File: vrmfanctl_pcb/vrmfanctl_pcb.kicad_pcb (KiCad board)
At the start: 2 copper layers, 27.9 x 33.3 mm, 14 parts, among them J1 SATA Power Male, J2 Pin header L-shape, J3 Pin socket L-shape, J4 Pin socket L-shape, Q1 2SC1740, Q2 2SC1740, Q3 2SC1740, U1 ATtiny85-20PU

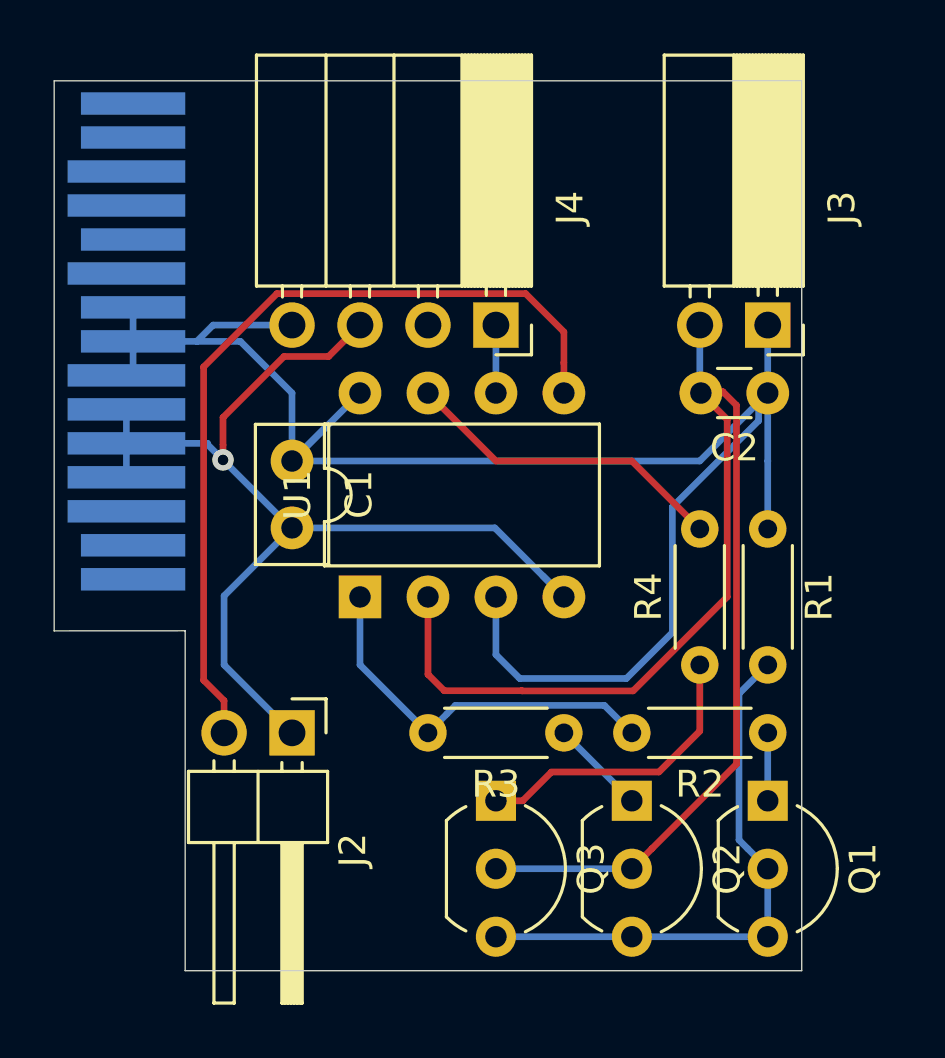
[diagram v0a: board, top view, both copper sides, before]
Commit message: update pcb layout
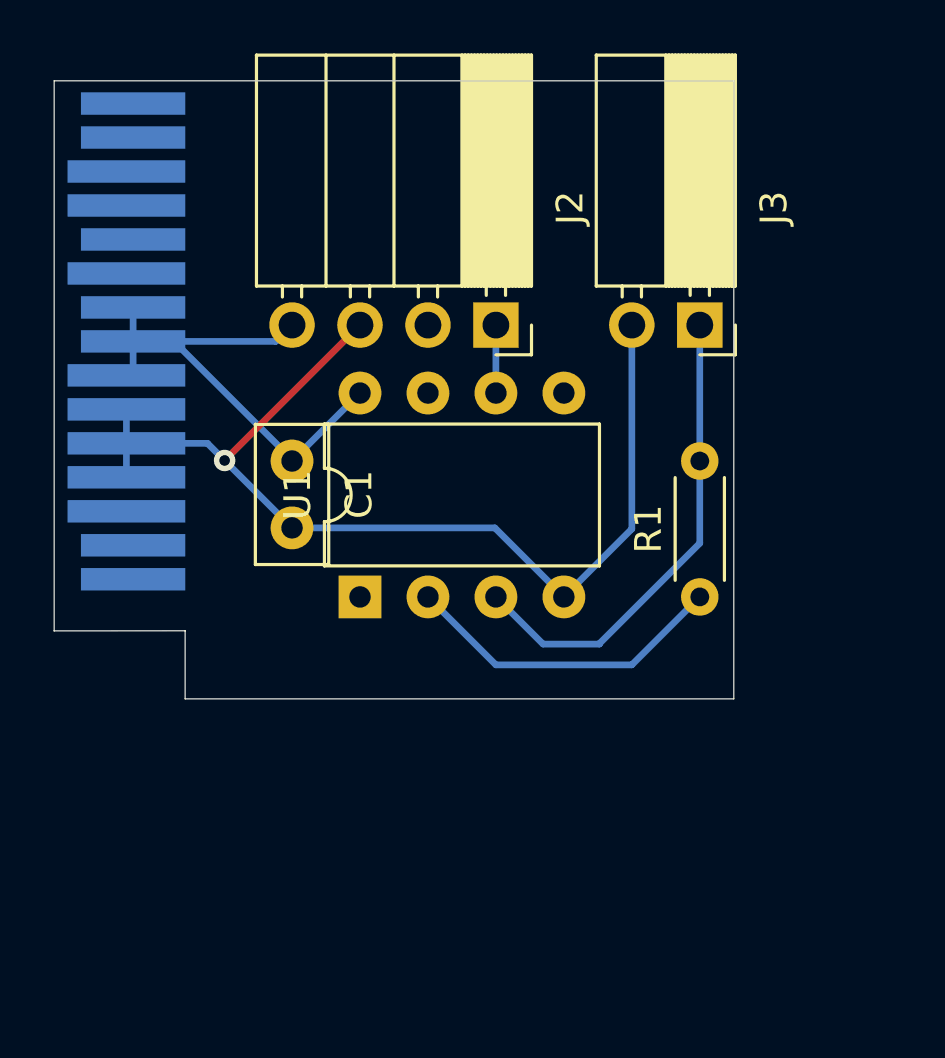
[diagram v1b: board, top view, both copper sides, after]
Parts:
- removed C2: 470p, Capacitor_THT:C_Disc_D3.0mm_W1.6mm_P2.50mm
- removed J4: Pin socket L-shape, Connector_PinSocket_2.54mm:PinSocket_1x04_P2.54mm_Horizontal
- removed Q1, Q2, Q3: 2SC1740, Package_TO_SOT_THT:TO-92_Inline_Wide
- removed R2, R3: 390k, Resistor_THT:R_Axial_DIN0204_L3.6mm_D1.6mm_P5.08mm_Horizontal
- removed R4: 20k, Resistor_THT:R_Axial_DIN0204_L3.6mm_D1.6mm_P5.08mm_Horizontal
- J2: value Pin header L-shape -> Pin socket L-shape; footprint Connector_PinHeader_2.54mm:PinHeader_1x02_P2.54mm_Horizontal -> Connector_PinSocket_2.54mm:PinSocket_1x04_P2.54mm_Horizontal
- R1: value 56k -> 3.9k
- moved J2 17.0 mm to (53.3, 50.8)
- moved R1 3.59 mm to (61.0, 61.0), turned to 90 degrees
- moved J3 2.54 mm to (61.0, 50.8)
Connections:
- J1 pad 1: Net-(J1-Pad1) -> (no net)
- J1 pad 10: Net-(J1-Pad10) -> (no net)
- J1 pad 11: Net-(J1-Pad11) -> (no net)
- J1 pad 12: Net-(J1-Pad12) -> (no net)
- J1 pad 13: Net-(J1-Pad13) -> (no net)
- J1 pad 14: Net-(J1-Pad14) -> (no net)
- J1 pad 15: Net-(J1-Pad15) -> (no net)
- J1 pad 2: Net-(J1-Pad2) -> (no net)
- J1 pad 3: Net-(J1-Pad3) -> (no net)
- J2 pad 1: GND -> /PWM
- J2 pad 2: /TX_RX -> (no net)
- J3 pad 1: VCC -> Net-(J3-Pad1)
- J3 pad 2: /D- -> GND
- R1 pad 1: VCC -> /THMPWR
- R1 pad 2: Net-(Q1-Pad2) -> Net-(J3-Pad1)
- U1 pad 1: /BDPWR10 -> (no net)
- U1 pad 2: /D- -> /THMPWR
- U1 pad 3: VCC -> Net-(J3-Pad1)
- U1 pad 5: /TX_RX -> (no net)
- U1 pad 7: /BDPWR200 -> (no net)
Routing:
- net /D-: track 52.1 -> 0.00 mm
- net VCC: track 69.6 -> 20.3 mm
- net /TX_RX: track 31.5 -> 0.00 mm
- net Net-(Q1-Pad2): track 21.2 -> 0.00 mm
- net Net-(J3-Pad1): track 0.00 -> 18.1 mm
- net /BDPWR10: track 14.6 -> 0.00 mm
- net /THMPWR: track 0.00 -> 12.3 mm
- net /BDPWR200: track 12.3 -> 0.00 mm
- net Net-(Q3-Pad1): track 11.2 -> 0.00 mm
- net Net-(Q2-Pad1): track 3.59 -> 0.00 mm
- net Net-(Q1-Pad1): track 2.54 -> 0.00 mm
- net GND: track 42.1 -> 39.6 mm
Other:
- board size 27.9 x 33.3 mm -> 25.4 x 23.1 mm
